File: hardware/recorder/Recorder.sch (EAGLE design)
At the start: 42 parts, among them T1 VN0109N3-G-ND, T2 IRF1404PBF, U1 DEV-16771_REDUCED_PINS, U2 MCP4822-E/P, U3 LM6132BIN, U4 Value, U5 L7808ABV, U6 L7908CV

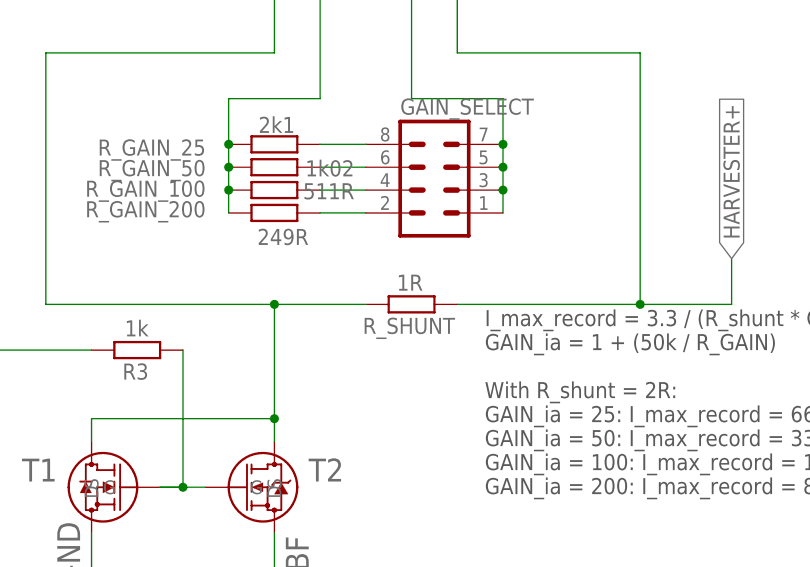
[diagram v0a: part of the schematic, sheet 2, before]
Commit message: Add minor changes to the hardware
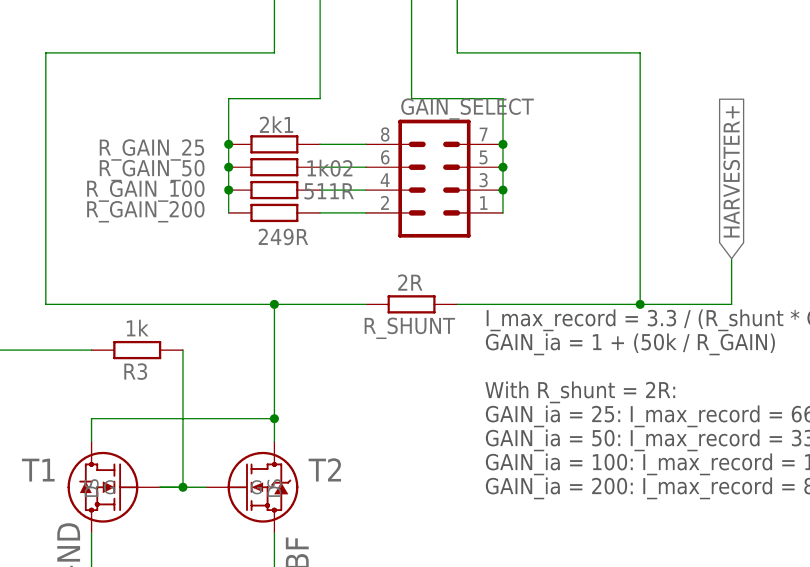
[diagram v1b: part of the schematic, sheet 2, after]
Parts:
- R_SHUNT: value 1R -> 2R
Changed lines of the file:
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@@
 <part name="SUPPLY20" library="supply2" library_urn="urn:adsk.eagle:library:372" deviceset="GND" device=""/>
 <part name="U4" library="INA121PA" deviceset="INA121PA" device="" value="Value"/>
-<part name="R_SHUNT" library="rcl" library_urn="urn:adsk.eagle:library:334" deviceset="R-EU_" device="0207/10" package3d_urn="urn:adsk.eagle:package:23491/2" value="1R"/>
+<part name="R_SHUNT" library="rcl" library_urn="urn:adsk.eagle:library:334" deviceset="R-EU_" device="0207/10" package3d_urn="urn:adsk.eagle:package:23491/2" value="2R"/>
 <part name="R_GAIN_25" library="rcl" library_urn="urn:adsk.eagle:library:334" deviceset="R-EU_" device="0207/10" package3d_urn="urn:adsk.eagle:package:23491/2" value="2k1"/>
 <part name="SUPPLY8" library="supply2" library_urn="urn:adsk.eagle:library:372" deviceset="GND" device=""/>
